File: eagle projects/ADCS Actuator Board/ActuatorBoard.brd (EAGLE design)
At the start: 91 x 91 mm, 260 parts, among them J4 OSTVN08A150, J5 OSTVN08A150, J6 OSTVN08A150, U10 TVS991, U11 BD6210F-E2, U12 ADS7841E_2K5, U13 ADS7841E_2K5, U15 TLV9051IDCKR, U16 BD6210F-E2, U17 DRV10970_MOTOR_DRIVERDRV10970, U18 DRV10970_MOTOR_DRIVERDRV10970, U19 TLV9051IDCKR, U20 DRV10970_MOTOR_DRIVERDRV10970, U21 TLV9051IDCKR, U22 BD6210F-E2, U23 TLV9051IDCKR, U24 TLV9051IDCKR, U25 ADS7841E_2K5, U26 TLV9051IDCKR, U27 ADS7841E_2K5, U28 TLV9051IDCKR, U29 TLV9051IDCKR, U30 TLV9051IDCKR, U31 TLV9051IDCKR, U32 TLV9051IDCKR, U4 ADS7841E_2K5, U6 TLV9051IDCKR, U7 TVS991, U8 TVS991, U9 ADS7841E_2K5

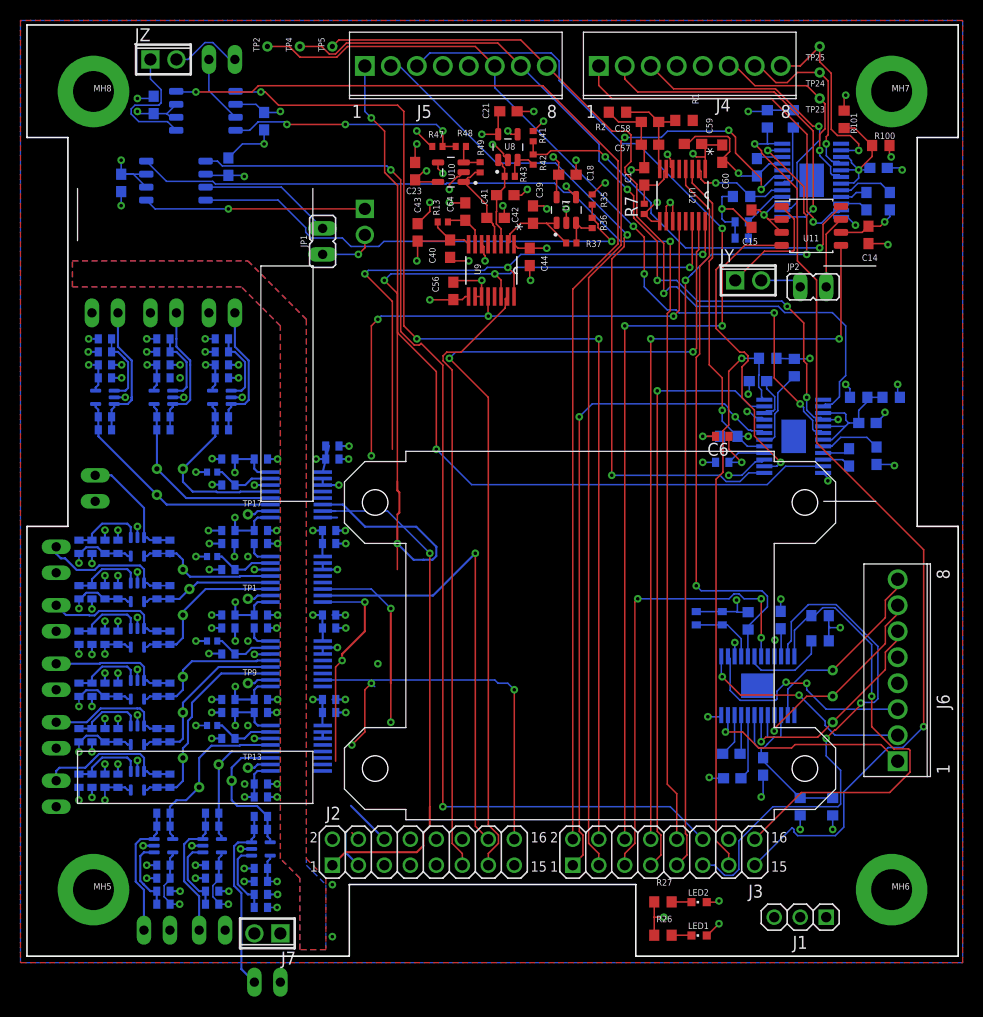
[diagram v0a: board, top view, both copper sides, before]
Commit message: fixed silkscreen fiasco
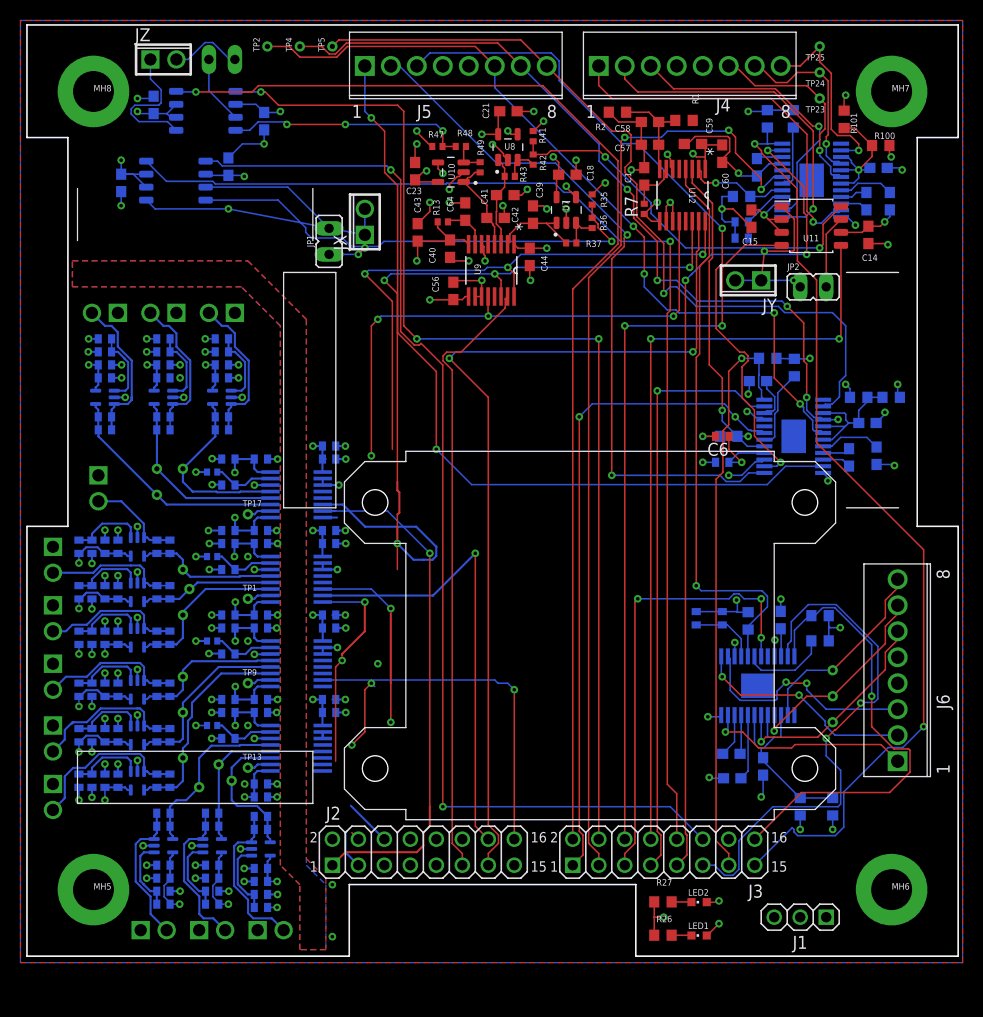
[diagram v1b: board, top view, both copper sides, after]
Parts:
- removed D1, D10, D11, D12, D13, D14, D15, D3, D5, D7, D8, D9: SFH2430, my_library:JP1Y_LED_SCREEN
- added J10, J11, J12, J13, J14, J15, J16, J17, J18, J8, J9: (no value), my_library:2POL254
- moved J7 61.5 mm to (13.3, 62.9), flipped to the bottom, turned to 0 degrees
- moved MX 2.31 mm to (25.1, 43.8)
- moved C79 1.31 mm to (29.5, 48.6)
- moved C80 1.31 mm to (29.5, 49.8)
- moved JP1 0.64 mm to (29.5, 69.8)
- flipped JX to the top, turned to 90 degrees
- turned JY to 180 degrees
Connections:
- removed net N$33: C100.1, D3.1, R31.1, U23.3
- removed net N$60: C98.1, D13.1, R64.1, U30.3
- new net N$23: C100.1, J7.2, R31.1, U23.3
- new net N$37: C98.1, J12.2, R64.1, U30.3
- net GND: now also J10.1, J11.1, J12.1, J13.1, J14.1, J15.1, J16.1, J17.1, J18.1, J7.1, J8.1, J9.1; no longer D1.2, D10.2, D11.2, D12.2, D13.2, D14.2, D15.2, D3.2, D5.2, D7.2, D8.2, D9.2
- net N$29: now also J8.2; no longer D1.1
- net N$35: now also J9.2; no longer D5.1
- net N$38: now also J15.2; no longer D7.1
- net N$44: now also J14.2; no longer D8.1
- net N$46: now also J13.2; no longer D9.1
- net N$49: now also J18.2; no longer D10.1
- net N$55: now also J17.2; no longer D11.1
- net N$57: now also J16.2; no longer D12.1
- net N$63: now also J11.2; no longer D14.1
- net N$65: now also J10.2; no longer D15.1
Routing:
- net N$60: track 18.6 -> 0.00 mm
- net N$37: track 0.00 -> 15.8 mm
- net N$23: track 0.00 -> 14.9 mm
- net N$33: track 13.6 -> 0.00 mm
- net OUT2_Y: track 4.07 -> 6.61 mm, vias 0 -> 1
- net +3V3: track 183.6 -> 186.1 mm
- net N$55: track 13.3 -> 15.6 mm
- net N$46: track 11.6 -> 9.33 mm
- net OUT2_X: track 5.66 -> 7.57 mm, vias 1 -> 2
- net N$63: track 13.7 -> 15.3 mm
- net N$49: track 15.0 -> 16.5 mm
- net N$29: track 13.8 -> 15.3 mm
- net N$57: track 12.7 -> 14.1 mm
- net N$35: track 13.6 -> 14.9 mm
- net OUT1_Y: track 11.8 -> 10.6 mm, vias 0 -> 1
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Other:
- board text added: "C72"
- board text added: "U15"
- board text added: "U19"
- board text added: "U21"
- board text added: "U23"
- board text added: "U24"
- board text added: "U26"
- board text added: "U28"
- board text added: "U29"
- board text added: "U30"
- board text added: "U31"
- board text added: "U32"
- board text added: "U6"
